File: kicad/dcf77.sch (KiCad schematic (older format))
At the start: 5 parts, among them U10 DCF77_Generic

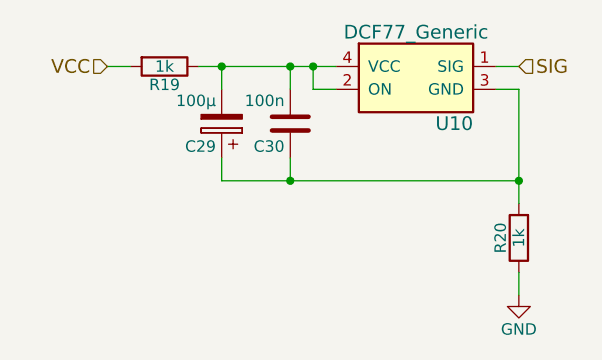
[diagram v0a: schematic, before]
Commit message: First routing
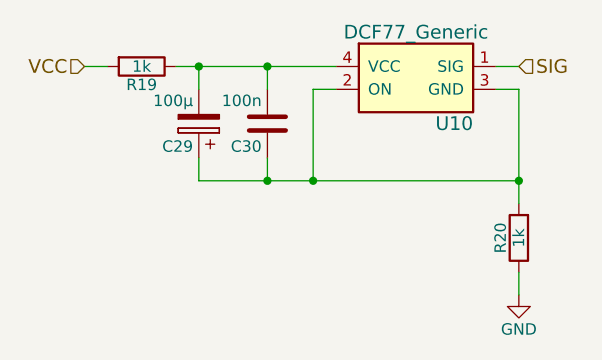
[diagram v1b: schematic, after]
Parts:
- C29, C30: footprint Capacitors_SMD:C_0805_HandSoldering -> Resistors_SMD:R_0805_HandSoldering
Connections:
- net at C29.2, C30.2, R19.1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: no longer U10.2 (ON)
- net at C29.1, C30.1, R20.2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: now also U10.2 (ON)
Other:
- moved on the sheet: C29, C30, R19
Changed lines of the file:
@@
 L C C30
 U 1 1 58DE81D9
-P 1850 1250
-F 0 "C30" H 1875 1350 50  0000 L CNN
-F 1 "100n" H 1875 1150 50  0000 L CNN
-F 2 "Capacitors_SMD:C_0805_HandSoldering" H 1888 1100 50  0001 C CNN
-F 3 "" H 1850 1250 50  0000 C CNN
-	1    1850 1250
+P 1750 1250
+F 0 "C30" H 1775 1350 50  0000 L CNN
+F 1 "100n" H 1775 1150 50  0000 L CNN
+F 2 "Resistors_SMD:R_0805_HandSoldering" H 1788 1100 50  0001 C CNN
+F 3 "" H 1750 1250 50  0000 C CNN
+	1    1750 1250
 	-1   0    0    1
 $EndComp
@@
 L CP C29
 U 1 1 58DE81E0
-P 1550 1250
-F 0 "C29" H 1575 1350 50  0000 L CNN
-F 1 "100µ" H 1575 1150 50  0000 L CNN
-F 2 "Capacitors_SMD:C_0805_HandSoldering" H 1588 1100 50  0001 C CNN
-F 3 "" H 1550 1250 50  0000 C CNN
-	1    1550 1250
+P 1450 1250
+F 0 "C29" H 1475 1350 50  0000 L CNN
+F 1 "100µ" H 1475 1150 50  0000 L CNN
+F 2 "Resistors_SMD:R_0805_HandSoldering" H 1488 1100 50  0001 C CNN
+F 3 "" H 1450 1250 50  0000 C CNN
+	1    1450 1250
 	-1   0    0    1
 $EndComp
@@
 L R R19
 U 1 1 58DE81E9
-P 1300 1000
-F 0 "R19" V 1380 1000 50  0000 C CNN
-F 1 "1k" V 1300 1000 50  0000 C CNN
-F 2 "Resistors_SMD:R_0805_HandSoldering" V 1230 1000 50  0001 C CNN
-F 3 "" H 1300 1000 50  0000 C CNN
-	1    1300 1000
+P 1200 1000
+F 0 "R19" V 1280 1000 50  0000 C CNN
+F 1 "1k" V 1200 1000 50  0000 C CNN
+F 2 "Resistors_SMD:R_0805_HandSoldering" V 1130 1000 50  0001 C CNN
+F 3 "" H 1200 1000 50  0000 C CNN
+	1    1200 1000
 	0    1    1    0
 $EndComp
@@
 	-1   0    0    1
 $EndComp
-Text HLabel 1050 1000 0    60   Input ~ 0
+Text HLabel 950  1000 0    60   Input ~ 0
 VCC
 Text HLabel 2850 1000 2    60   Input ~ 0
@@
 	2750 1100 2850 1100
 Wire Wire Line
-	1450 1000 2050 1000
-Wire Wire Line
-	1950 1000 1950 1100
+	1350 1000 2050 1000
 Wire Wire Line
 	1950 1100 2050 1100
-Connection ~ 1950 1000
 Wire Wire Line
-	1550 1100 1550 1000
-Connection ~ 1550 1000
+	1450 1100 1450 1000
+Connection ~ 1450 1000
 Wire Wire Line
-	1850 1100 1850 1000
-Connection ~ 1850 1000
+	1750 1100 1750 1000
+Connection ~ 1750 1000
 Wire Wire Line
 	2750 1000 2850 1000
@@
 	2850 1900 2850 2000
 Wire Wire Line
-	1550 1400 1550 1500
+	1450 1400 1450 1500
 Wire Wire Line
-	1550 1500 2850 1500
-Wire Wire Line
-	1850 1400 1850 1500
-Connection ~ 1850 1500
+	1750 1400 1750 1500
+Connection ~ 1750 1500
 Wire Wire Line
 	2850 1100 2850 1600
 Connection ~ 2850 1500
 Wire Wire Line
-	1050 1000 1150 1000
+	950  1000 1050 1000
+Wire Wire Line
+	1950 1500 1950 1100
+Wire Wire Line
+	1450 1500 2850 1500
+Connection ~ 1950 1500
 $EndSCHEMATC
